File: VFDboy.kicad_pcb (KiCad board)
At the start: 2 copper layers, 139.5 x 60 mm, 108 parts, among them J1 AVR-ISP-6, J2 USB_C_Receptacle_USB2.0, J3 Micro_SD_Card_Det, J4 TagConnect_TC2030_SWD, Q1 FS8205A, Q2 S9015, Q3 AO3401A, Q4 AO3401A, Q5 S9015, Q6 2N7002, Q7 AO3401A, Q9 AO3401A, SW1 RIGHT, SW2 A, SW3 DOWN, SW4 UP, SW5 LEFT, SW6 B, SW8 POWER, U1 ATmega32U4-MU, U2 SSD1306_VFD, U3 SY7088, U4 XC6206P332MR, U5 DW01+G, U6 TP4054, U7 SRV05-4, U8 STM32L151C8Tx, U9 BQ34Z100, Y1 16MHz

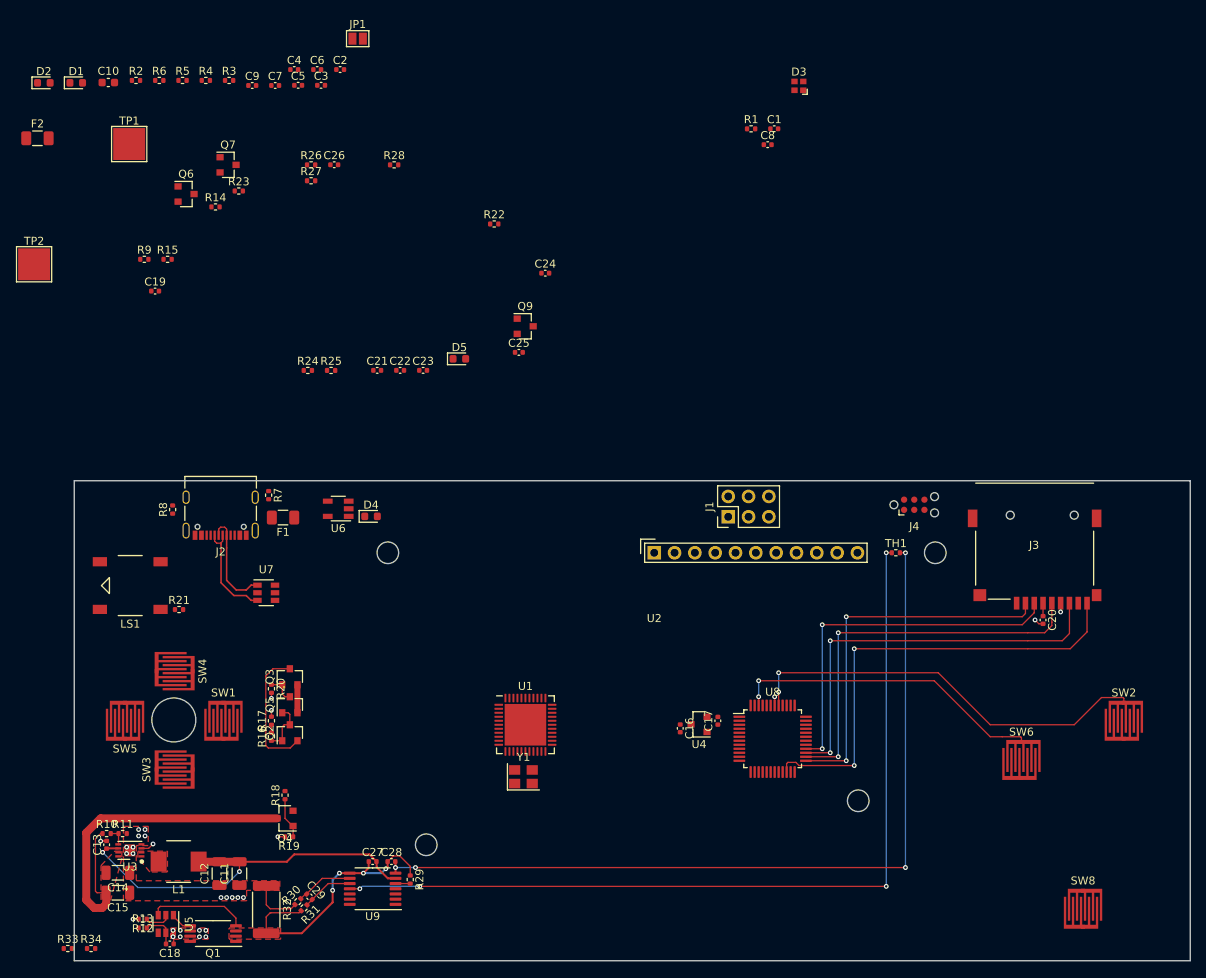
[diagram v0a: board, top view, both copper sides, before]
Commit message: Partially routed
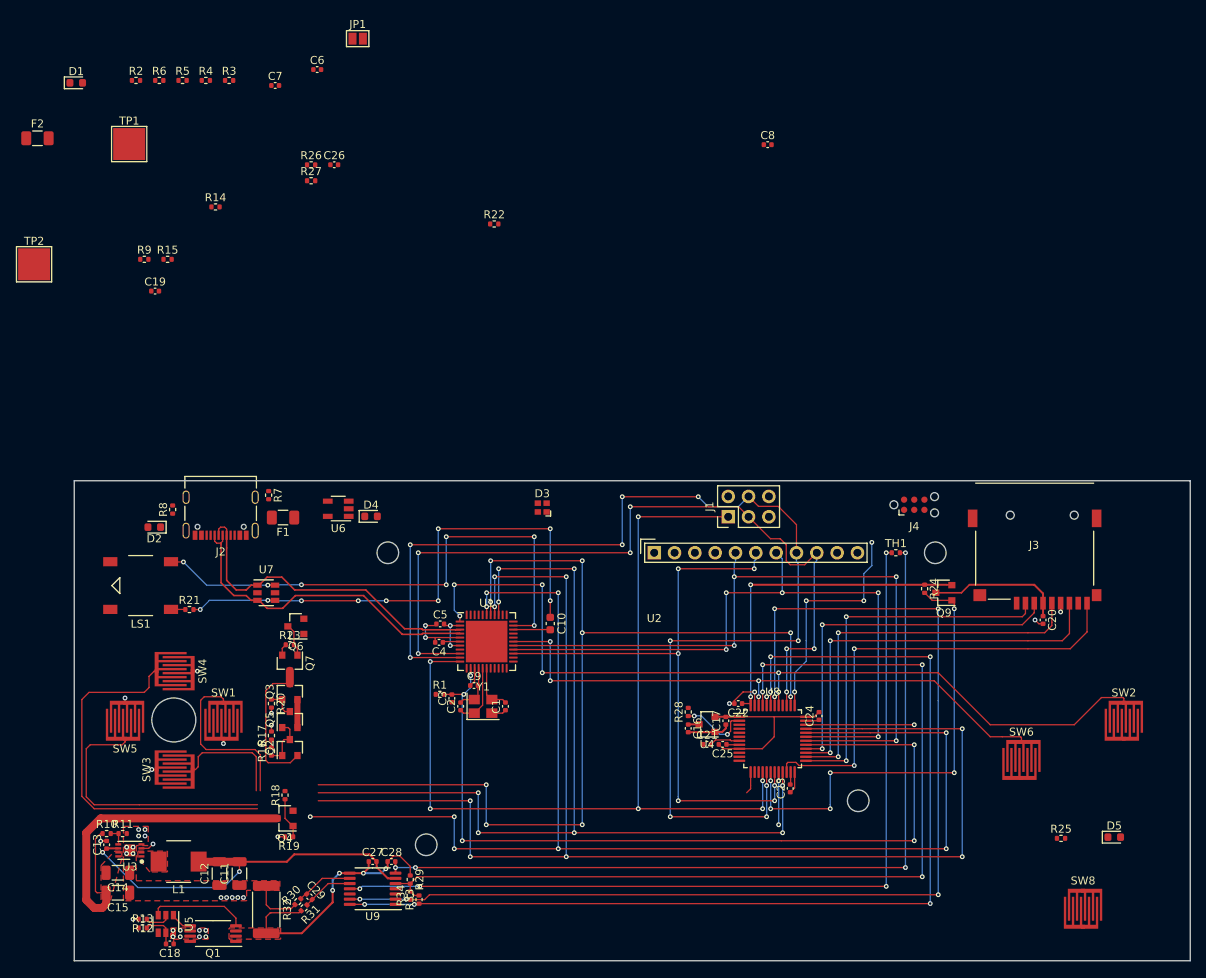
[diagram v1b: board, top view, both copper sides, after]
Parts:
- moved R25 108.4 mm to (225.8, 144.7)
- moved D5 101.4 mm to (232.5, 144.6)
- moved C10 87.3 mm to (162.0, 117.8), turned to 270 degrees
- moved R24 81.8 mm to (208.8, 113.5), turned to 270 degrees
- moved C2 81.0 mm to (150.8, 128.2), turned to 90 degrees
- moved R1 80.7 mm to (148.2, 126.7)
- moved C9 80.0 mm to (152.5, 125.6)
- moved C1 79.6 mm to (156.4, 128.2), turned to 90 degrees
- moved C3 78.4 mm to (149.7, 127.2), turned to 90 degrees
- moved R28 77.6 mm to (179.2, 128.9), turned to 90 degrees
- moved C4 73.9 mm to (148.1, 120.2), turned to 180 degrees
- moved C5 69.6 mm to (148.2, 117.9)
- moved C23 69.5 mm to (192.0, 138.4), turned to 90 degrees
- moved C24 65.1 mm to (195.6, 129.4), turned to 90 degrees
- moved Q7 62.8 mm to (129.4, 122.8), turned to 270 degrees
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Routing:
- net /RIGHT: track 0.00 -> 193.4 mm, vias 0 -> 8
- net /DOWN: track 0.00 -> 173.3 mm, vias 0 -> 9
- net /UP: track 0.00 -> 165.2 mm, vias 0 -> 8
- net /LEFT: track 0.00 -> 157.8 mm, vias 0 -> 9
- net /MOSI: track 0.00 -> 147.4 mm, vias 0 -> 10
- net /Power/SCL: track 1.09 -> 142.2 mm, vias 1 -> 6
- net /Power/SDA: track 0.00 -> 129.4 mm, vias 0 -> 6
- net /Power/GAUGE_EN: track 1.84 -> 120.0 mm, vias 0 -> 4
- net /MISO: track 0.00 -> 116.0 mm, vias 0 -> 6
- net /~RST: track 0.00 -> 106.5 mm, vias 0 -> 5
- net /SCK: track 0.00 -> 100.9 mm, vias 0 -> 7
- net /~OLEDRST: track 0.00 -> 91.3 mm, vias 0 -> 4
- net /~CS: track 0.00 -> 85.1 mm, vias 0 -> 5
- net /~DC: track 0.00 -> 76.8 mm, vias 0 -> 6
- net +3V3: track 0.00 -> 67.8 mm, vias 0 -> 2
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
